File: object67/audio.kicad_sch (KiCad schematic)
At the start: 51 parts, among them IC1 AK4493SEQ, IC2 TAA5242IRGER, IC3 LMK1C1104PWR, U1 RCJ-2223, Y1 22.5792M, Y2 24.576M

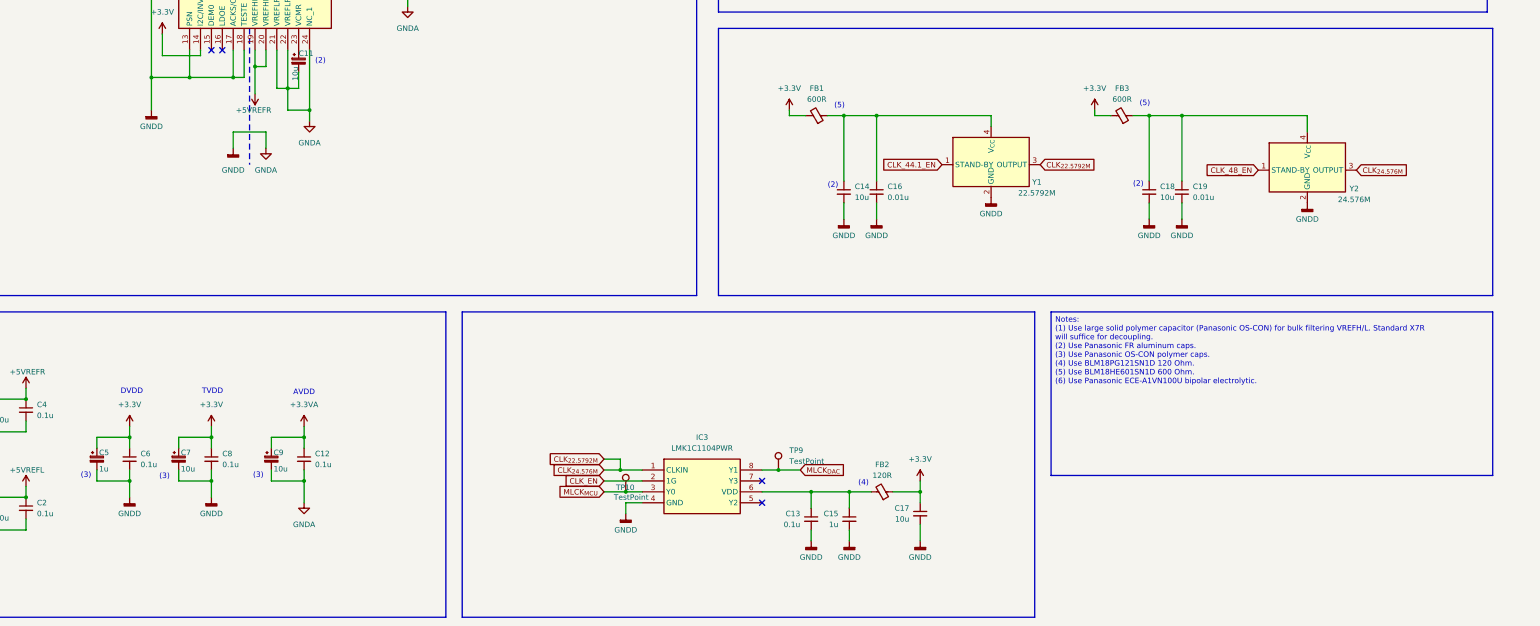
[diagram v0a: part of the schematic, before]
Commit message: Finished layout
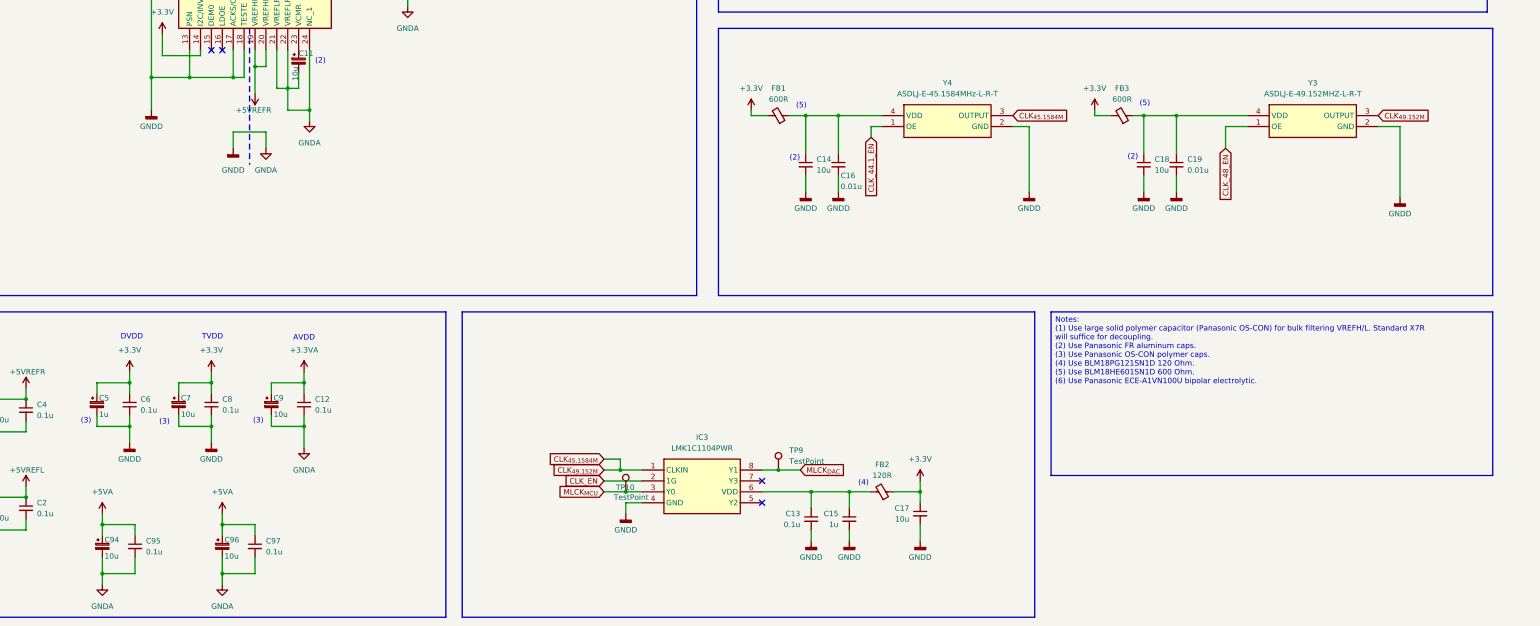
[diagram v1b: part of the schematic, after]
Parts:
- removed Y1: 22.5792M, object67:Oscillator_SMD_NDK_NZ2520SDA-4Pin_2.5x2.0mm, symbol object67:NSC5083D-22.5792M
- removed Y2: 24.576M, object67:Oscillator_SMD_NDK_NZ2520SDA-4Pin_2.5x2.0mm, symbol object67:NSC5083D-24.576M
- added C94, C96: 10u, Capacitor_SMD:CP_Elec_5x5.3, symbol Device:C_Polarized_Small
- added C95, C97: 0.1u, Capacitor_SMD:C_0603_1608Metric, symbol Device:C_Small
- added Y3: ASDLJ-E-49.152MHZ-L-R-T, object67:ASDLJE49152MHZLRT, symbol object67:ASDLJ-E-49.152MHZ-L-R-T
- added Y4: ASDLJ-E-45.1584MHz-L-R-T, object67:ASDLJE451584MHzLRT, symbol object67:ASDLJ-E-45.1584MHz-L-R-T
- C1: footprint (none) -> Capacitor_THT:CP_Radial_D8.0mm_P5.00mm
- C10, C11: footprint (none) -> Capacitor_THT:CP_Radial_D5.0mm_P2.00mm
- C12, C13, C2, C4, C8: footprint (none) -> Capacitor_SMD:C_0603_1608Metric
- C14, C18, C20, C21, C7, C9: footprint (none) -> Capacitor_SMD:CP_Elec_4x5.3
- C15, C17, C23, C25, C26, C5, C58: footprint (none) -> Capacitor_SMD:C_1206_3216Metric
- C16, C19, C22, C6: footprint (none) -> Capacitor_SMD:C_0402_1005Metric
- C3: footprint (none) -> Capacitor_THT:CP_Radial_D8.0mm_P3.50mm
- FB1, FB2, FB3: footprint (none) -> Inductor_SMD:L_0603_1608Metric
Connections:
- net +5VA: now also C94.1, C95.1, C96.1, C97.1
- net CLK_44.1_EN: now also Y4.1 (OE)
- net CLK_48_EN: now also Y3.1 (OE)
- net GNDA: now also C94.2, C95.2, C96.2, C97.2, Y3.2 (GND), Y4.2 (GND)
- net at C14.1, C16.1, FB1.1: now also Y4.4 (VDD)
- net at C18.1, C19.1, FB3.1: now also Y3.4 (VDD)
- net CLK_{22.5792M} renamed CLK_{45.1584M}
- net CLK_{45.1584M}: now also Y3.3 (OUTPUT), Y4.3 (OUTPUT)
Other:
- moved on the sheet: C12, C14, C16, C18, C19, C5, C6, C7, C8, C9, FB1

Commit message: Start layout
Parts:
- R1, R2: footprint (none) -> Resistor_SMD:R_0402_1005Metric
- R33: footprint (none) -> Resistor_SMD:R_1206_3216Metric
- TP10, TP11, TP12, TP13, TP14, TP15, TP16, TP17, TP5, TP6, TP7, TP8, TP9: footprint (none) -> TestPoint:TestPoint_Pad_D2.0mm
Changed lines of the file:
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@@
 			)
 		)
-		(property "Footprint" ""
+		(property "Footprint" "TestPoint:TestPoint_Pad_D2.0mm"
 			(at 151.13 124.46 0)
 			(effects
@@
 			)
 		)
-		(property "Footprint" ""
+		(property "Footprint" "TestPoint:TestPoint_Pad_D2.0mm"
 			(at 266.7 34.29 0)
 			(effects
@@
 			)
 		)
-		(property "Footprint" ""
+		(property "Footprint" "TestPoint:TestPoint_Pad_D2.0mm"
 			(at 241.3 247.65 0)
 			(effects
@@
 			)
 		)
-		(property "Footprint" ""
+		(property "Footprint" "Resistor_SMD:R_0402_1005Metric"
 			(at 43.18 254 0)
 			(effects
@@
 			)
 		)
-		(property "Footprint" ""
+		(property "Footprint" "TestPoint:TestPoint_Pad_D2.0mm"
 			(at 156.21 101.6 0)
 			(effects
@@
 			)
 		)
-		(property "Footprint" ""
+		(property "Footprint" "TestPoint:TestPoint_Pad_D2.0mm"
 			(at 151.13 99.06 0)
 			(effects
@@
 			)
 		)
-		(property "Footprint" ""
+		(property "Footprint" "TestPoint:TestPoint_Pad_D2.0mm"
 			(at 158.75 127 0)
 			(effects
@@
 			)
 		)
-		(property "Footprint" ""
+		(property "Footprint" "TestPoint:TestPoint_Pad_D2.0mm"
 			(at 205.74 252.73 0)
 			(effects
@@
 			)
 		)
-		(property "Footprint" ""
+		(property "Footprint" "Resistor_SMD:R_0402_1005Metric"
 			(at 43.18 231.14 0)
 			(effects
@@
 			)
 		)
-		(property "Footprint" ""
+		(property "Footprint" "TestPoint:TestPoint_Pad_D2.0mm"
 			(at 264.16 31.75 0)
 			(effects
@@
 			)
 		)
-		(property "Footprint" ""
+		(property "Footprint" "TestPoint:TestPoint_Pad_D2.0mm"
 			(at 68.5535 101.6 0)
 			(effects
@@
 			)
 		)
-		(property "Footprint" ""
+		(property "Footprint" "Resistor_SMD:R_1206_3216Metric"
 			(at 256.54 118.11 0)
 			(effects
@@
 			)
 		)
-		(property "Footprint" ""
+		(property "Footprint" "TestPoint:TestPoint_Pad_D2.0mm"
 			(at 76.2 106.68 0)
 			(effects
@@
 			)
 		)
-		(property "Footprint" ""
+		(property "Footprint" "TestPoint:TestPoint_Pad_D2.0mm"
 			(at 72.39 104.14 0)
 			(effects
@@
 			)
 		)
-		(property "Footprint" ""
+		(property "Footprint" "TestPoint:TestPoint_Pad_D2.0mm"
 			(at 80.01 109.22 0)
 			(effects
@@
 			)
 		)
-		(property "Footprint" ""
+		(property "Footprint" "TestPoint:TestPoint_Pad_D2.0mm"
 			(at 269.24 36.83 0)
 			(effects
